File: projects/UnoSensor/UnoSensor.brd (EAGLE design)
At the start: 53.8 x 53.3 mm, 8 parts

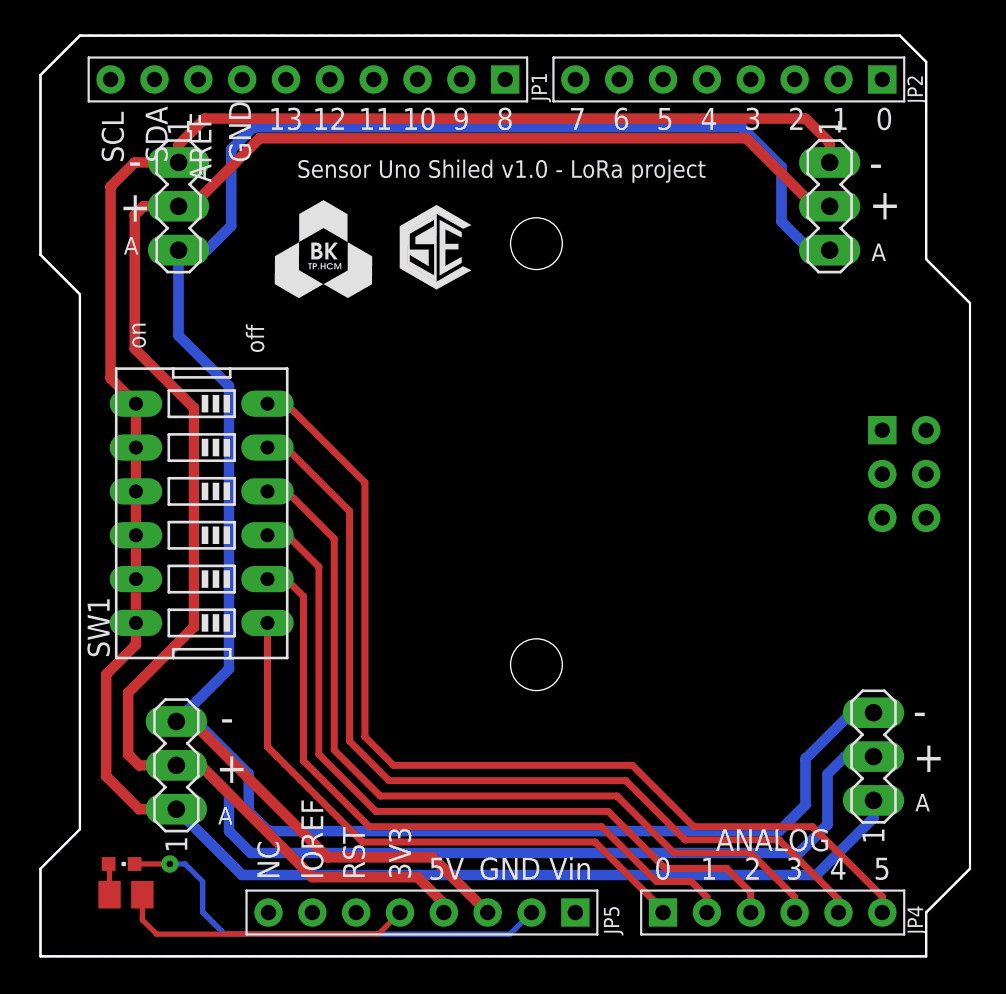
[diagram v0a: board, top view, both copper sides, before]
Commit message: init
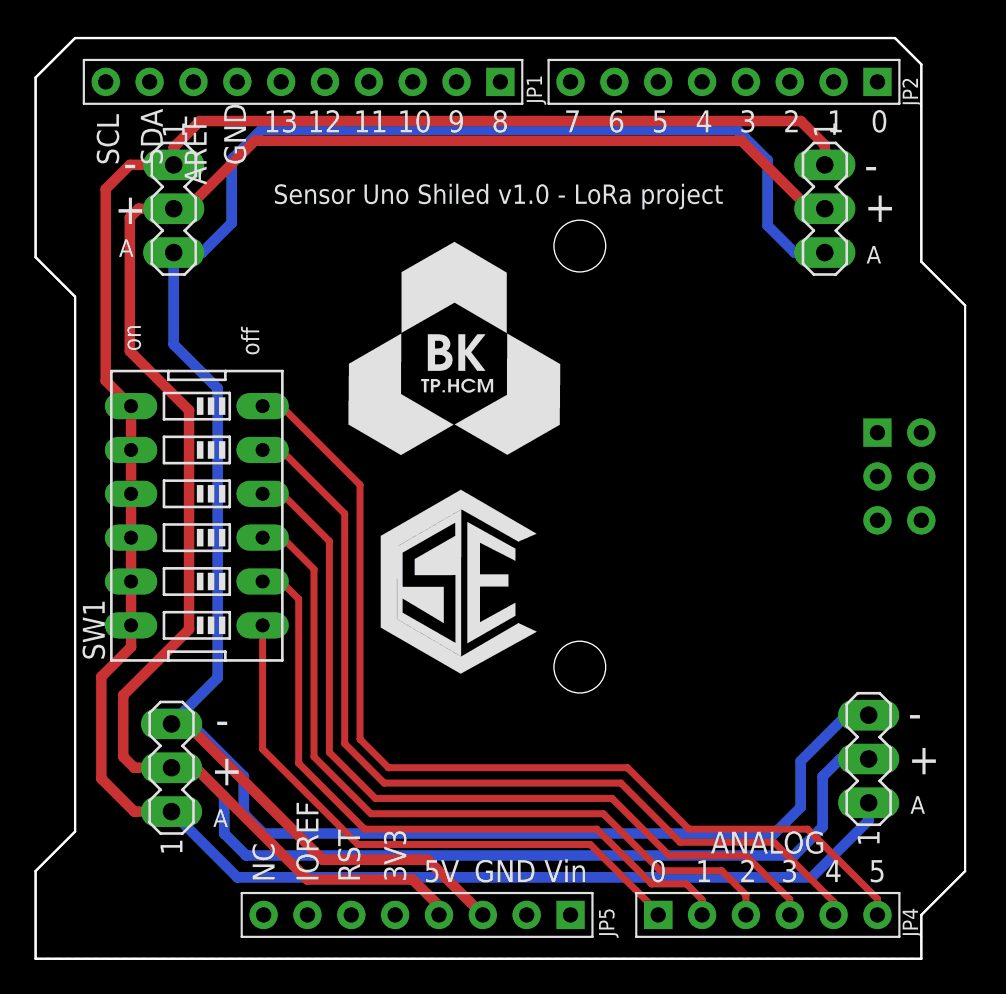
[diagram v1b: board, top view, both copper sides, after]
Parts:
- removed LED1: (no value), adafruit:CHIPLED_0603
- removed R1: 330, adafruit:M0805
- moved SW1 0.31 mm to (9.42, 25.8)
- moved U5 0.31 mm to (20.9, 26.8)
- moved SV1 0.31 mm to (7.95, 11.2)
- moved SV2 0.31 mm to (8.08, 43.5)
- moved SV4 0.31 mm to (48.3, 11.7)
- moved SV3 0.31 mm to (45.8, 43.5)
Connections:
- removed net N$2: R1.2, U5.22
- removed net N$8: LED1.A, R1.1
- removed net N$9: LED1.C, U5.25
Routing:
- net N$9: track 26.2 -> 0.00 mm, vias 1 -> 0
- net N$2: track 17.2 -> 0.00 mm
- net N$8: track 1.80 -> 0.00 mm
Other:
- board text added: "Design by Le Phuong Nam Phone No. 0981662961 BKU - CSE - 1512067"
- board text removed: "433MHZ"
- board text removed: "868MHZ"
- board text removed: "915MHZ"

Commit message: init
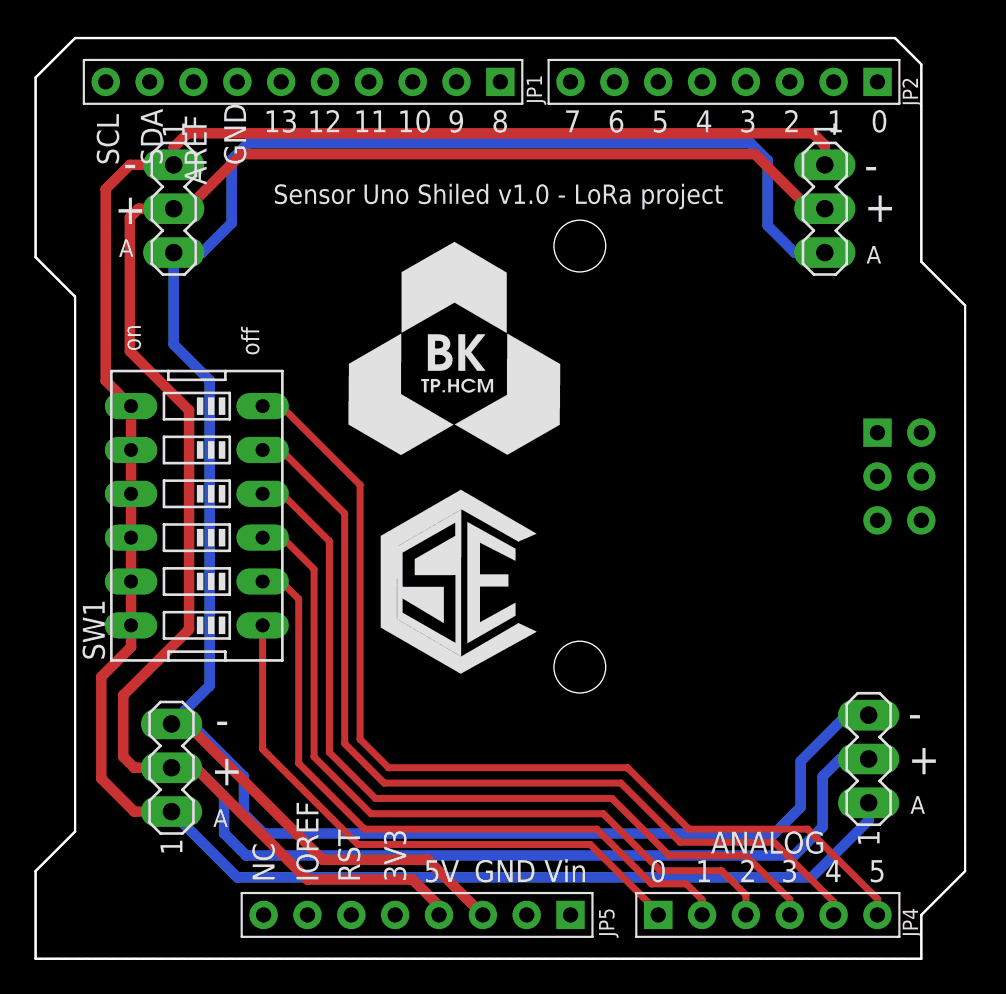
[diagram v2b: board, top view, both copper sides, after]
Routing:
- net GND-0V: track 148.9 -> 147.8 mm
- net 5V: track 148.1 -> 147.5 mm
- net DATA: track 130.3 -> 129.7 mm
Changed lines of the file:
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@@
 <drawing>
 <settings>
-<setting alwaysvectorfont="yes"/>
+<setting alwaysvectorfont="no"/>
 <setting keepoldvectorfont="yes"/>
 <setting verticaltext="up"/>
@@
 <wire x1="4.144771875" y1="44.680634375" x2="5.541771875" y2="46.077634375" width="0.6096" layer="1"/>
 <wire x1="5.541771875" y1="46.077634375" x2="8.081771875" y2="46.077634375" width="0.6096" layer="1"/>
-<wire x1="44.403771875" y1="48.617634375" x2="9.605771875" y2="48.617634375" width="0.6096" layer="1"/>
-<wire x1="9.605771875" y1="48.617634375" x2="8.081771875" y2="47.093634375" width="0.6096" layer="1"/>
+<wire x1="45.114971875" y1="47.906434375" x2="8.894571875" y2="47.906434375" width="0.6096" layer="1"/>
+<wire x1="8.894571875" y1="47.906434375" x2="8.081771875" y2="47.093634375" width="0.6096" layer="1"/>
 <wire x1="8.081771875" y1="46.077634375" x2="8.081771875" y2="47.093634375" width="0.6096" layer="1"/>
 <wire x1="45.800771875" y1="47.220634375" x2="45.800771875" y2="46.077634375" width="0.6096" layer="1"/>
-<wire x1="45.800771875" y1="47.220634375" x2="44.403771875" y2="48.617634375" width="0.6096" layer="1"/>
+<wire x1="45.800771875" y1="47.220634375" x2="45.114971875" y2="47.906434375" width="0.6096" layer="1"/>
 <wire x1="7.954771875" y1="8.612634375" x2="11.764771875" y2="4.802634375" width="0.6096" layer="16"/>
 <wire x1="11.764771875" y1="4.802634375" x2="45.038771875" y2="4.802634375" width="0.6096" layer="16"/>
@@
 <contactref element="SV4" pad="2"/>
 <wire x1="8.081771875" y1="43.537634375" x2="8.843771875" y2="43.537634375" width="0.6096" layer="1"/>
-<wire x1="12.780771875" y1="47.474634375" x2="40.974771875" y2="47.474634375" width="0.6096" layer="1"/>
-<wire x1="40.974771875" y1="47.474634375" x2="44.911771875" y2="43.537634375" width="0.6096" layer="1"/>
+<wire x1="12.006071875" y1="46.699934375" x2="41.749471875" y2="46.699934375" width="0.6096" layer="1"/>
+<wire x1="41.749471875" y1="46.699934375" x2="44.911771875" y2="43.537634375" width="0.6096" layer="1"/>
 <wire x1="44.911771875" y1="43.537634375" x2="45.800771875" y2="43.537634375" width="0.6096" layer="1"/>
-<wire x1="8.843771875" y1="43.537634375" x2="12.780771875" y2="47.474634375" width="0.6096" layer="1"/>
+<wire x1="8.843771875" y1="43.537634375" x2="12.006071875" y2="46.699934375" width="0.6096" layer="1"/>
 <wire x1="8.081771875" y1="43.537634375" x2="6.049771875" y2="43.537634375" width="0.6096" layer="1"/>
 <wire x1="6.049771875" y1="43.537634375" x2="5.541771875" y2="43.029634375" width="0.6096" layer="1"/>
@@
 <wire x1="44.0443625" y1="40.997634375" x2="42.492675" y2="42.549321875" width="0.6096" layer="16"/>
 <wire x1="42.492675" y1="42.549321875" x2="42.492675" y2="46.33773125" width="0.6096" layer="16"/>
-<wire x1="42.492675" y1="46.33773125" x2="40.720771875" y2="48.109634375" width="0.6096" layer="16"/>
-<wire x1="40.720771875" y1="48.109634375" x2="13.170915625" y2="48.109634375" width="0.6096" layer="16"/>
+<wire x1="42.492675" y1="46.33773125" x2="41.495471875" y2="47.334934375" width="0.6096" layer="16"/>
+<wire x1="41.495471875" y1="47.334934375" x2="12.396215625" y2="47.334934375" width="0.6096" layer="16"/>
 <wire x1="11.4394" y1="46.37811875" x2="11.4394" y2="42.7042625" width="0.6096" layer="16"/>
 <wire x1="11.4394" y1="42.7042625" x2="9.732771875" y2="40.997634375" width="0.6096" layer="16"/>
 <wire x1="9.732771875" y1="40.997634375" x2="8.081771875" y2="40.997634375" width="0.6096" layer="16"/>
-<wire x1="13.170915625" y1="48.109634375" x2="11.4394" y2="46.37811875" width="0.6096" layer="16"/>
-<wire x1="10.634728125" y1="33.123634375" x2="8.081771875" y2="35.676590625" width="0.6096" layer="16"/>
+<wire x1="12.396215625" y1="47.334934375" x2="11.4394" y2="46.37811875" width="0.6096" layer="16"/>
+<wire x1="10.164828125" y1="33.593534375" x2="8.081771875" y2="35.676590625" width="0.6096" layer="16"/>
 <wire x1="8.081771875" y1="40.997634375" x2="8.081771875" y2="35.676590625" width="0.6096" layer="16"/>
-<wire x1="10.634728125" y1="16.372590625" x2="7.954771875" y2="13.692634375" width="0.6096" layer="16"/>
-<wire x1="10.634728125" y1="33.123634375" x2="10.634728125" y2="16.372590625" width="0.6096" layer="16"/>
+<wire x1="10.164828125" y1="15.902690625" x2="7.954771875" y2="13.692634375" width="0.6096" layer="16"/>
+<wire x1="10.164828125" y1="33.593534375" x2="10.164828125" y2="15.902690625" width="0.6096" layer="16"/>
 <wire x1="7.954771875" y1="13.692634375" x2="9.097771875" y2="13.692634375" width="0.6096" layer="16"/>
 <wire x1="12.145771875" y1="10.644634375" x2="12.145771875" y2="8.485634375" width="0.6096" layer="16"/>
